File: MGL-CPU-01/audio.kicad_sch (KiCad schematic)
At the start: 40 parts, among them P5 Headphones, U3 IR3R53N

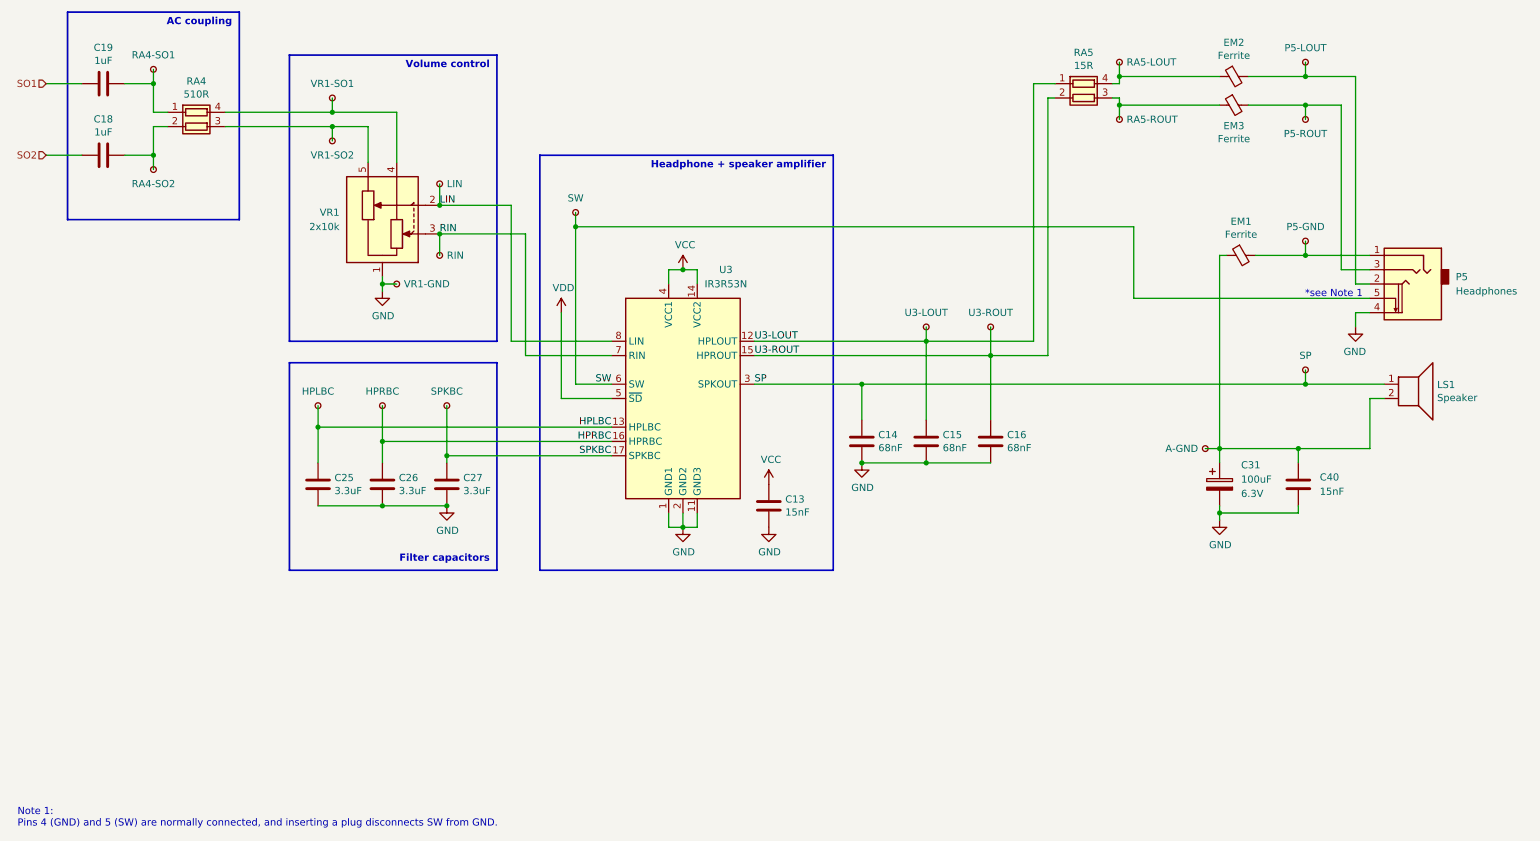
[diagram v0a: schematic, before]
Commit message: Update to latest KiCad
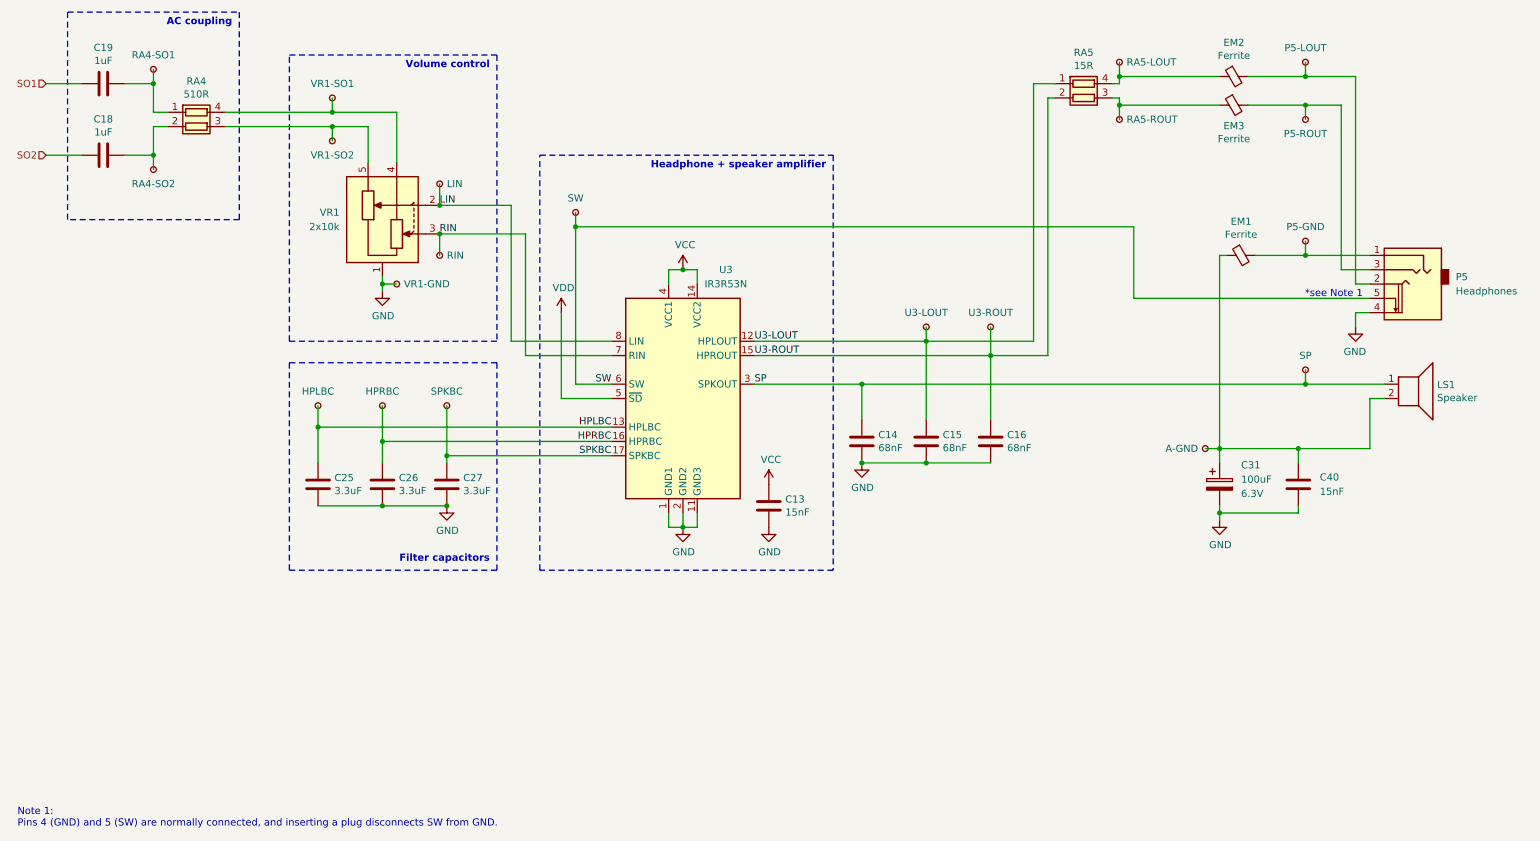
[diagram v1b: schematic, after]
